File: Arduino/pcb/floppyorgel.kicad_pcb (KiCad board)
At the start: 2 copper layers, 50 x 50 mm, 56 parts, among them J1 VCC_Power_Select, J2 Floppy-Bus, J3 MAX485 Socket, J4 Floppy-Bus, J5 Buck-Converter-5V, J6 Buck-Converter-12V, J7 Floppy-Power, J8 IBM_PC_Floppy_IDC, J9 FTDI, Q1 IRLML2060, Q2 IRLML2060, Q3 IRLML2060, SW1 Bus Address Select, SW2 Reset Button, U1 4021, U2 ATMEGA328P-AU, U3 24LC64, U4 74HC595, Y1 20 Mhz Crystal

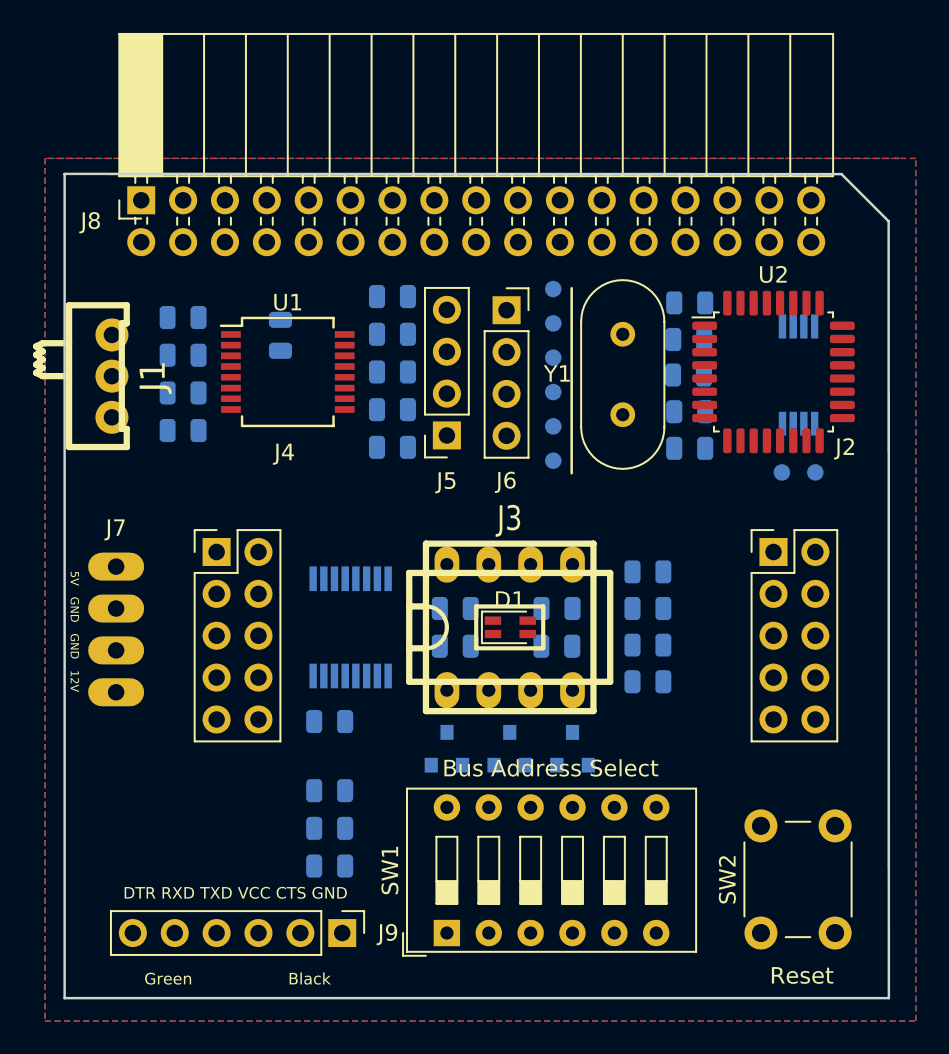
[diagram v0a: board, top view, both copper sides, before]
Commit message: pcb: some routing
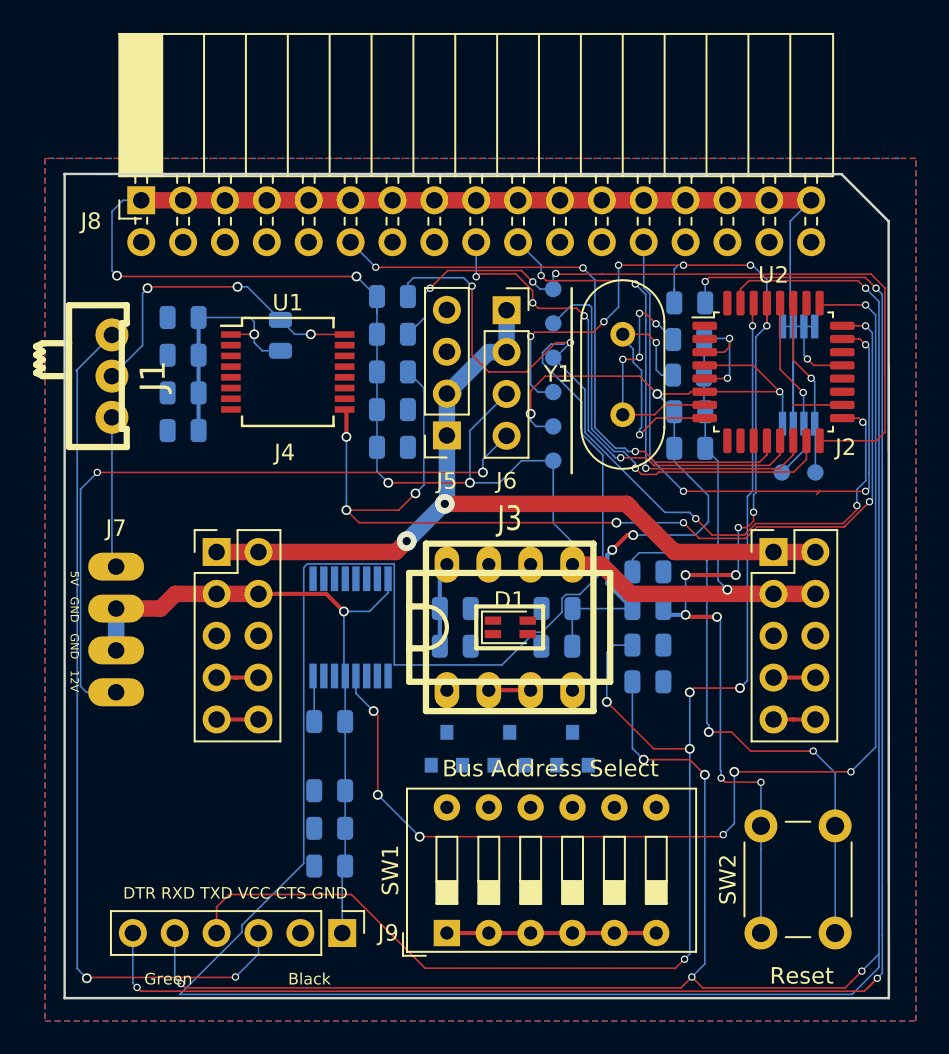
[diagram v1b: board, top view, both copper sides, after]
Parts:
- turned C7 to 0 degrees
- turned R1 to 180 degrees
- turned R16 to 0 degrees
- turned R5 to 0 degrees
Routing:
- net Net-(J9-Pad5): track 0.00 -> 234.9 mm, vias 0 -> 6
- net GND: track 0.00 -> 222.9 mm, vias 0 -> 10
- net Net-(C3-Pad2): track 0.00 -> 104.0 mm, vias 0 -> 4
- net VCC: track 0.00 -> 95.4 mm, vias 0 -> 8
- net Net-(J9-Pad4): track 0.00 -> 86.5 mm, vias 0 -> 6
- net /MCU/RESET: track 0.00 -> 77.0 mm, vias 0 -> 14
- net /Led/LATCH_LED: track 0.00 -> 72.9 mm, vias 0 -> 7
- net /Floppy/LATCH_ADDR: track 0.00 -> 64.4 mm, vias 0 -> 7
- net /Bus/BUS_POWER: track 0.00 -> 54.2 mm, vias 0 -> 2
- net /5V_ISP: track 0.00 -> 52.4 mm, vias 0 -> 2
- net /Floppy/SCK: track 0.00 -> 49.8 mm, vias 0 -> 5
- net /Floppy/MISO: track 0.00 -> 46.0 mm, vias 0 -> 3
- net /Floppy/12V_BUS: track 0.00 -> 42.8 mm, vias 0 -> 2
- net /Floppy/TRK00: track 0.00 -> 38.1 mm, vias 0 -> 3
- net /Floppy/DRIVE_SELECT: track 0.00 -> 37.1 mm, vias 0 -> 3
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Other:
- net class Default: clearance 0.2 -> 0.1; trace_width 0.25 -> 0.1; via_dia 0.6 -> 0.45; via_drill 0.4 -> 0.3
- rule pad_to_mask_clearance: 0.2 -> 0.1
- rule solder_mask_min_width: 0.25 -> 0.1
- rule trace_clearance: 0.2 -> 0.1
- rule trace_min: 0.2 -> 0.1
- rule via_min_drill: 0.3 -> 0.2
- rule via_min_size: 0.4 -> 0.45
